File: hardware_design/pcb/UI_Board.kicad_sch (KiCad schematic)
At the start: 30 parts, among them J2 Thonkiconn, J3 Thonkiconn, J4 Thonkiconn, J5 Thonkiconn, J6 Thonkiconn, J7 Thonkiconn, SW1 SW_Rotary_1x4, SW2 SW_SPST, SW3 RotaryEncoder_Switch, SW4 SW_SPST, SW5 SW_Rotary_1x8, U8 MC14532B

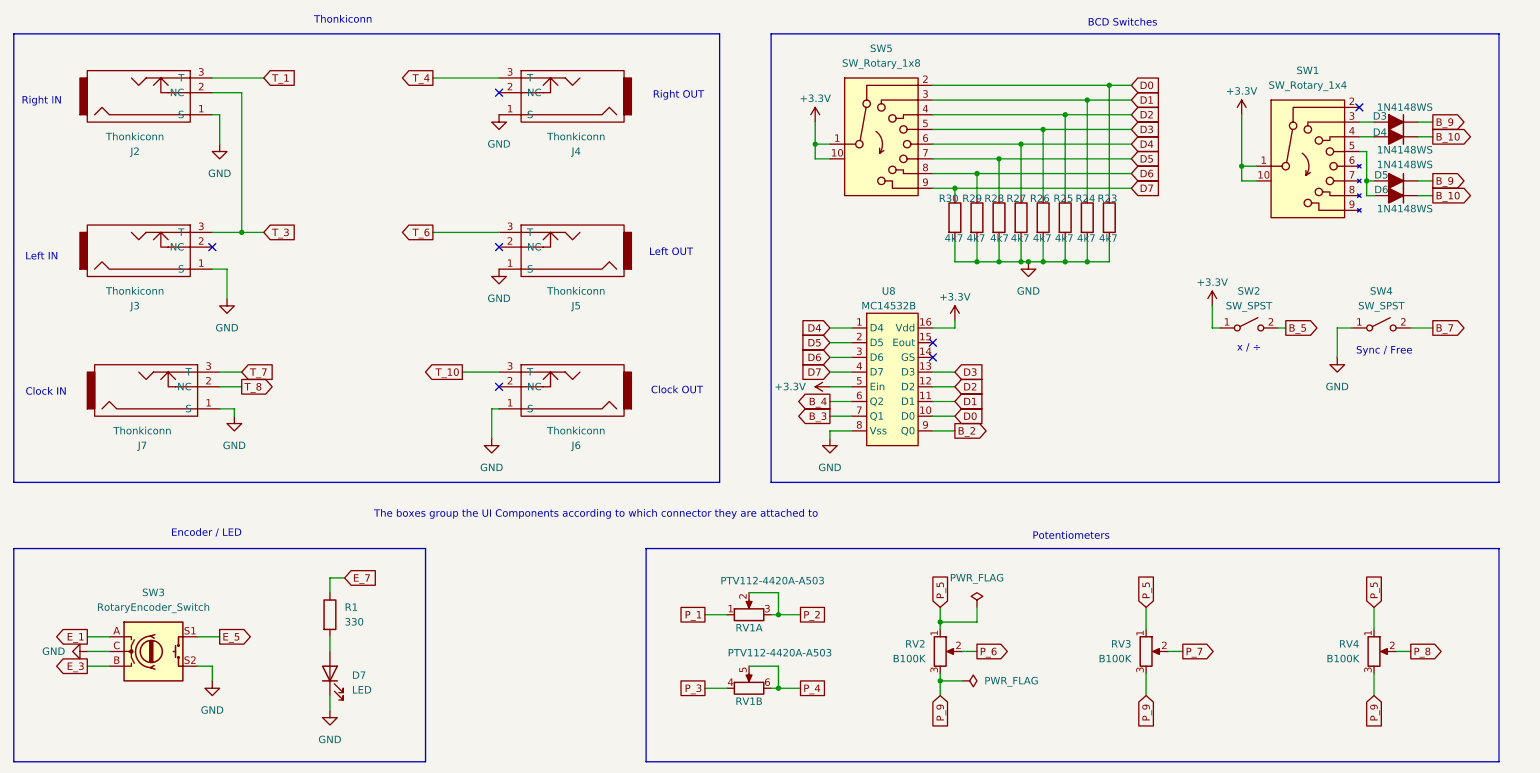
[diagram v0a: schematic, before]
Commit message: Rev 2 schematic & circuit board
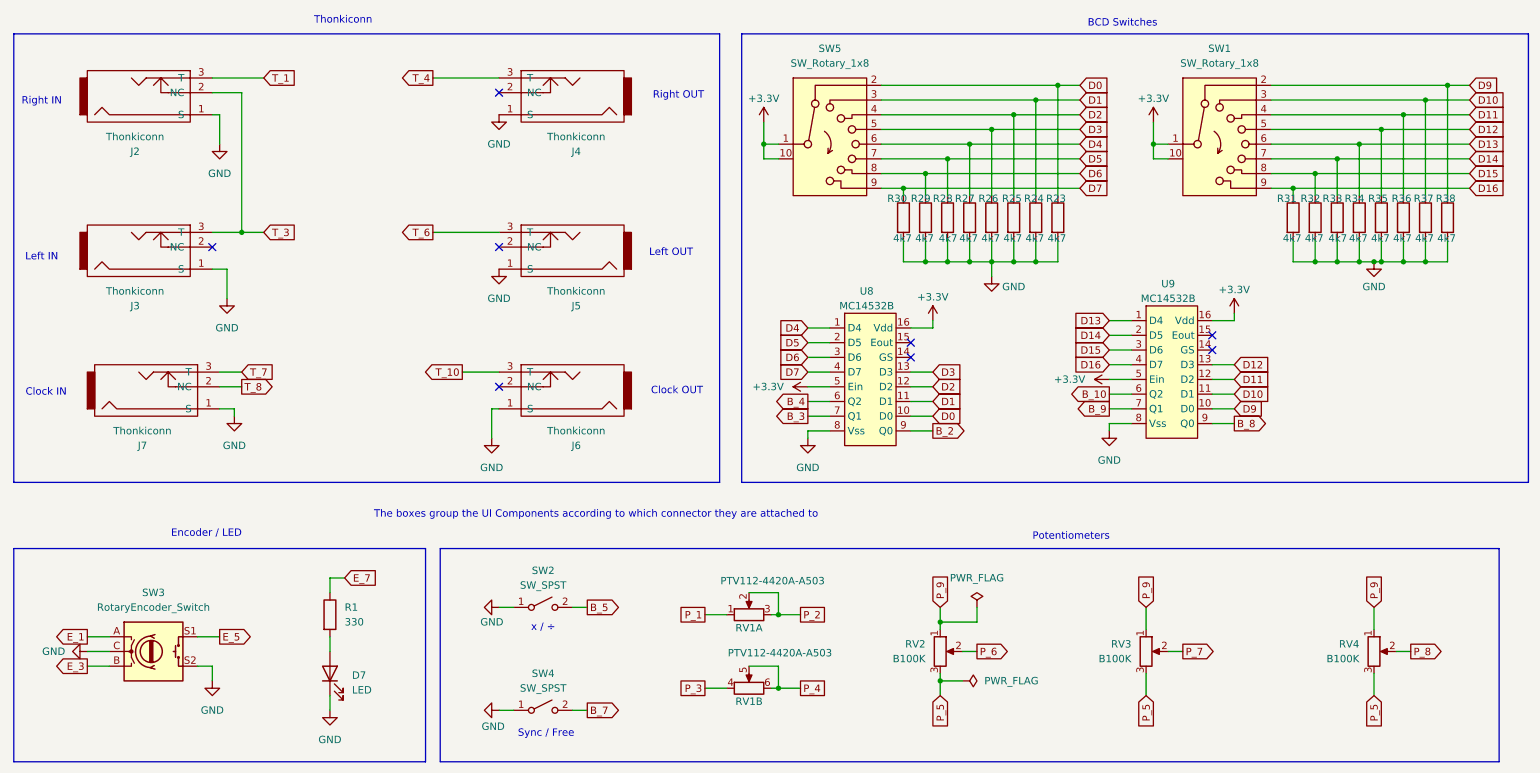
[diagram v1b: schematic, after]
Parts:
- removed D3, D4, D5, D6: 1N4148WS, Diode_SMD_AKL:D_SOD-323, symbol Diode_AKL:1N4148WS
- removed SW1: SW_Rotary_1x4, DSP_CodecBoards:ALPS Alpine 8-Way rotary switch SRBV Series, symbol DSP_CodecBoards:SW_Rotary_1x4
- added R31, R32, R33, R34, R35, R36, R37, R38: 4k7, Resistor_SMD_AKL:R_0603_1608Metric_Pad1.05x0.95mm_HandSolder, symbol Device:R
- added SW1: SW_Rotary_1x8, DSP_CodecBoards:ALPS Alpine 8-Way rotary switch SRBV Series, symbol DSP_CodecBoards:SW_Rotary_1x8
- added U9: MC14532B, Package_SO:SOIC-16_3.9x9.9mm_P1.27mm, symbol DSP_CodecBoards:MC14532
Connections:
- net +3.3V: now also SW1.1, SW1.10, U9.16 (Vdd), U9.5 (Ein); no longer SW2.1 (A)
- net B_10: now also U9.6 (Q2)
- net B_9: now also U9.7 (Q1)
- net GND: now also SW2.1 (A), R31.2, R32.2, R33.2, R34.2, R35.2, R36.2, R37.2, R38.2, U9.8 (Vss)
- net P_5: now also RV2.3, RV3.3, RV4.3; no longer RV2.1, RV3.1, RV4.1
- net P_9: now also RV2.1, RV3.1, RV4.1; no longer RV2.3, RV3.3, RV4.3
- new net B_8: U9.9 (Q0)
- new net D10: R37.1, SW1.3, U9.11 (D1)
- new net D11: R36.1, SW1.4, U9.12 (D2)
- new net D12: R35.1, SW1.5, U9.13 (D3)
- new net D13: R34.1, SW1.6, U9.1 (D4)
- new net D14: R33.1, SW1.7, U9.2 (D5)
- new net D15: R32.1, SW1.8, U9.3 (D6)
- new net D16: R31.1, SW1.9, U9.4 (D7)
- new net D9: R38.1, SW1.2, U9.10 (D0)
- no-connect marks 7 -> 8
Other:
- moved on the sheet: R23, R24, R25, R26, R27, R28, R29, R30, SW2, SW4, SW5, U8
